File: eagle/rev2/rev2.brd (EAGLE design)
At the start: 160 x 100 mm, 101 parts

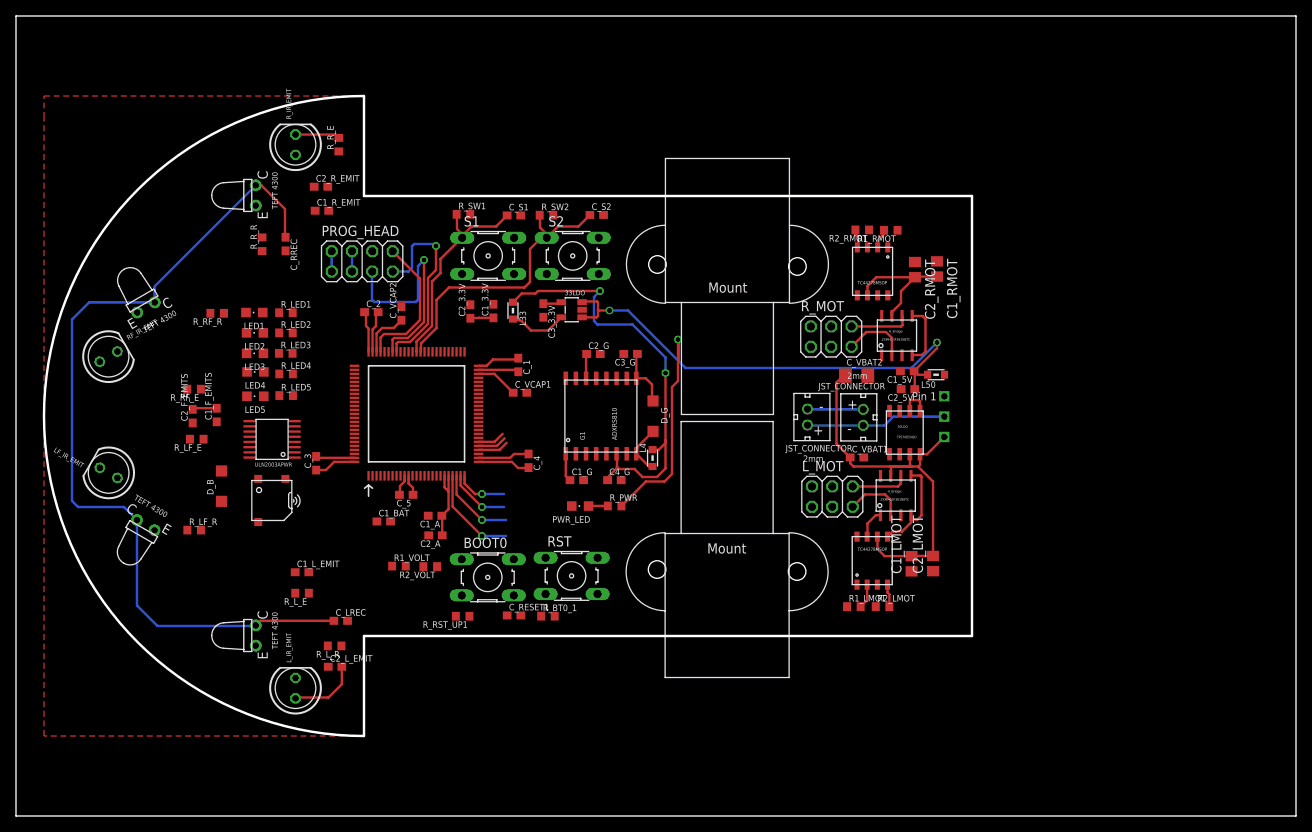
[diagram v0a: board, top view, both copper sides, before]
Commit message: Clean directory
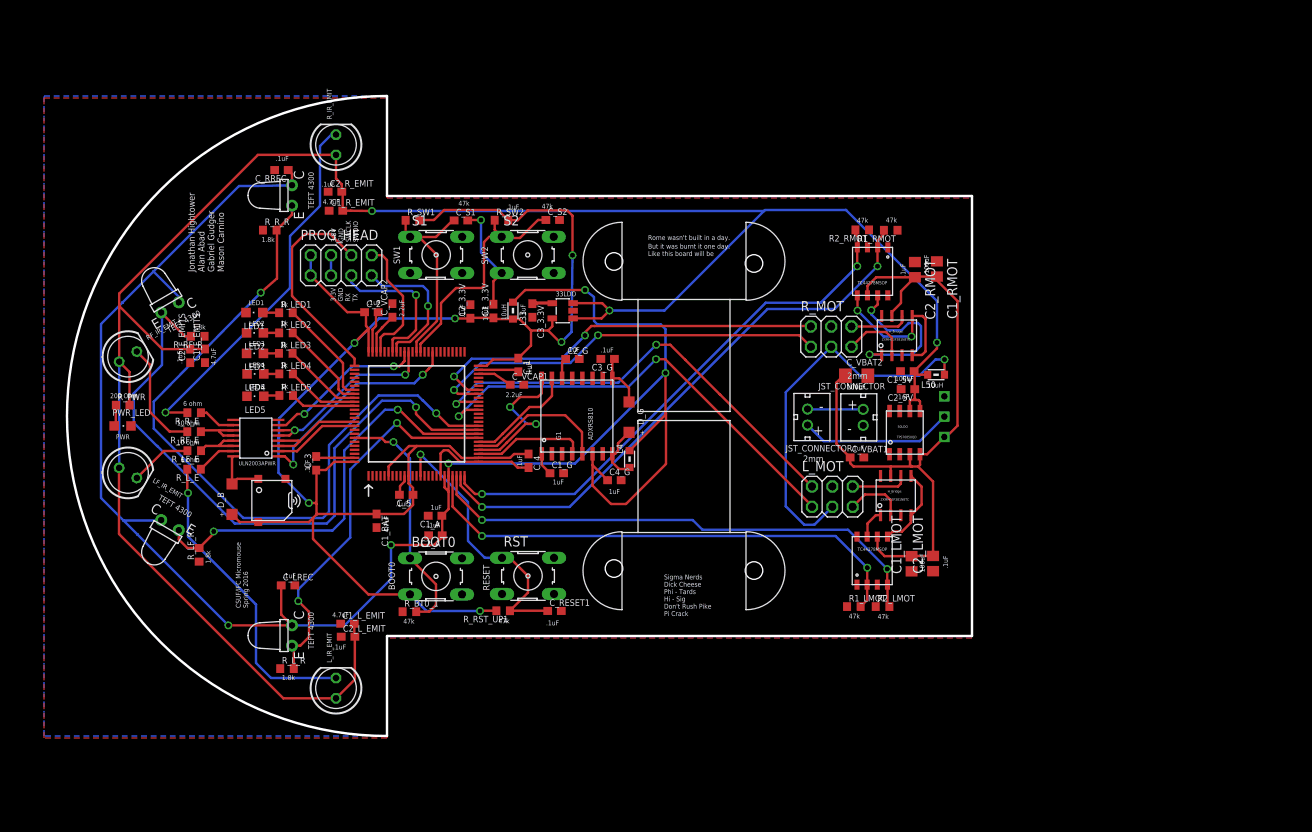
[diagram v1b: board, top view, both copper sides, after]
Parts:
- removed R1_VOLT: 20k, resistor:R0603
- removed R2_VOLT: 10k, resistor:R0603
- removed U$5: MOTOR, mounts:MOTOR_MOUNT
- added U$1: MOTOR, mounts:MOTOR_MOUNT
- U$3: value STM32F769VG-1 -> STM32F746VG
- moved R_PWR 62.8 mm to (13.3, 51.4)
- moved PWR_LED 58.1 mm to (13.3, 48.8), turned to 270 degrees
- moved R_R_E 38.1 mm to (22.3, 50.4), turned to 180 degrees
- moved R_L_E 20.6 mm to (22.3, 43.4)
- moved R_BT0_1 17.3 mm to (49.2, 25.5)
- moved C_RREC 9.26 mm to (33.2, 80.7), turned to 180 degrees
- moved C1_L_EMIT 8.59 mm to (41.4, 24.0)
- moved C_LREC 7.94 mm to (34.0, 28.8)
- moved C1_F_EMITS 7.55 mm to (23.6, 57.5)
- moved C2_F_EMITS 7.54 mm to (21.8, 57.5)
- moved C_S1 6.65 mm to (55.6, 74.4)
- moved R_L_R 6.60 mm to (33.9, 18.4), turned to 0 degrees
- moved S1 6.50 mm to (52.5, 70.1)
- moved BOOT0 6.47 mm to (52.5, 30.0)
- moved R_SW1 6.42 mm to (49.6, 74.5)
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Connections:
- removed net VOLTMETER: R1_VOLT.1, R2_VOLT.2, U$3.15
- net GND: no longer R2_VOLT.1
- net LENCA: now also U$3.39; no longer U$3.41
- net LENCB: now also U$3.41; no longer U$3.39
- net RENCA: now also U$3.43; no longer U$3.44
- net RENCB: now also U$3.44; no longer U$3.43
- net V_BAT: no longer R1_VOLT.2
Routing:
- net 3.3V: track 37.5 -> 215.6 mm, vias 0 -> 6
- net 5V: track 104.9 -> 269.4 mm
- net RIGHT_REC: track 0.00 -> 93.1 mm, vias 0 -> 2
- net RF_REC: track 0.00 -> 82.0 mm, vias 0 -> 1
- net A3.3V: track 171.6 -> 236.9 mm, vias 2 -> 5
- net RPWMA: track 10.2 -> 71.7 mm, vias 1 -> 2
- net RPWMB: track 8.78 -> 67.1 mm, vias 1 -> 2
- net LENCB: track 0.00 -> 57.8 mm, vias 0 -> 2
- net LENCA: track 0.00 -> 57.6 mm, vias 0 -> 2
- net LF_REC: track 0.00 -> 52.6 mm, vias 0 -> 2
- net LPWMB: track 12.8 -> 65.0 mm, vias 1 -> 2
- net RENCA: track 0.00 -> 51.3 mm, vias 0 -> 2
- net RENCB: track 0.00 -> 51.2 mm, vias 0 -> 2
- net LEFT_REC: track 0.00 -> 48.9 mm, vias 0 -> 2
- net LPWMA: track 15.1 -> 64.0 mm, vias 1 -> 2
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- added copper zone on layer 16, net GND
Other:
- board size 160 x 100 mm -> 113.1 x 80 mm
- board text added: "+"
- board text added: ".1uF"
- board text added: "1.8k"
- board text added: "10 ohm"
- board text added: "100uF"
- board text added: "10uF"
- board text added: "10uH"
- board text added: "1k"
- board text added: "1uF"
- board text added: "2.2uF"
- board text added: "200 Ohm"
- board text added: "3.3V GND RX TX"
- board text added: "3.3V GND SWCLK SWDIO"
- board text added: "4.7uF"
- board text added: "47k"
- board text added: "6 ohm"
- board text added: "BOOT0"
- board text added: "But it was burnt it one day. Like this board will be"
- board text added: "CSUF/IFC Micromouse Spring 2016"
- board text added: "Jonathan Hightower Alan Abad Gabriel Gudger Mason Carnino"
- board text added: "LED1"
- board text added: "LED2"
- board text added: "LED3"
- board text added: "LED4"
- board text added: "LED5"
- board text added: "PWR"
- board text added: "RESET"
- board text added: "Rome wasn't built in a day."
- board text added: "SW1"
- board text added: "SW2"
- board text added: "Sigma Nerds Dick Cheese Phi - Tards Hi - Sig Don't Rush Pike Pi Crack"
